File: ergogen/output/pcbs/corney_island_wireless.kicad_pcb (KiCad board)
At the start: 2 copper layers, 133.8 x 91.7 mm, 75 parts

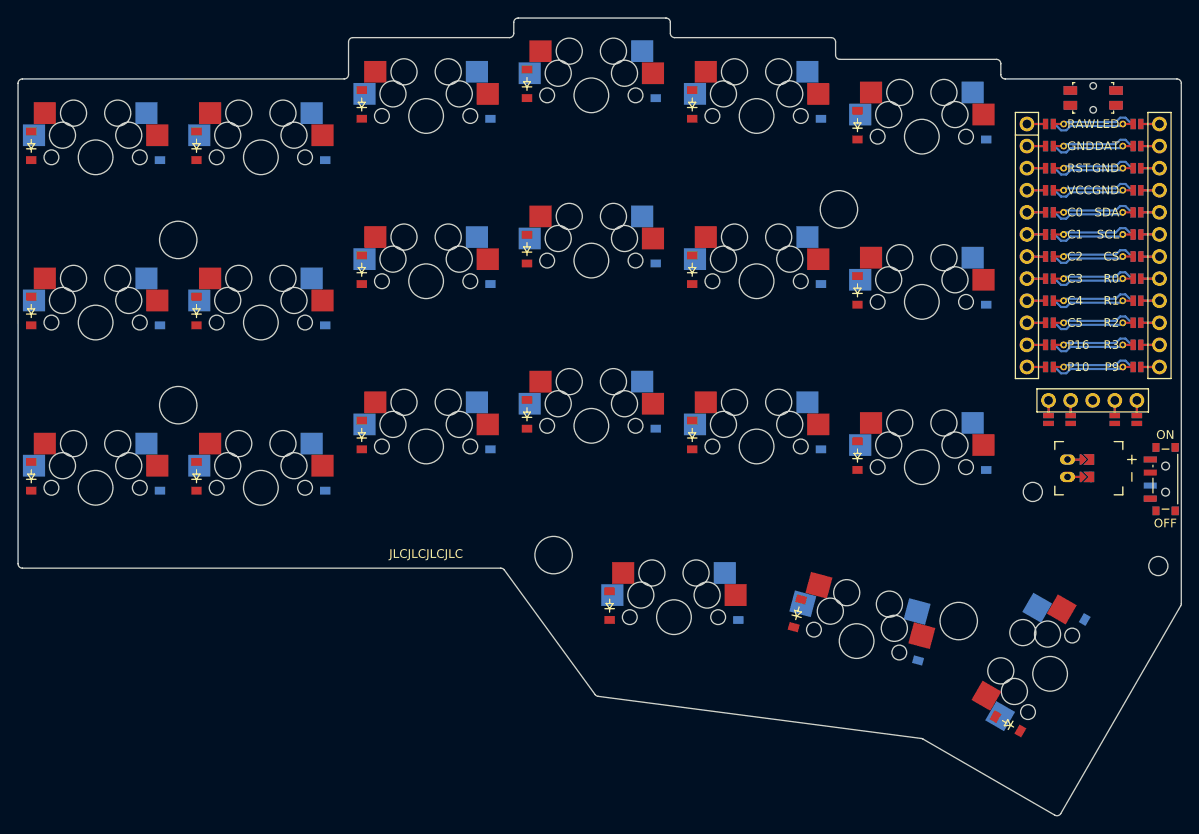
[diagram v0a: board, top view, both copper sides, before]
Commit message: Update assets
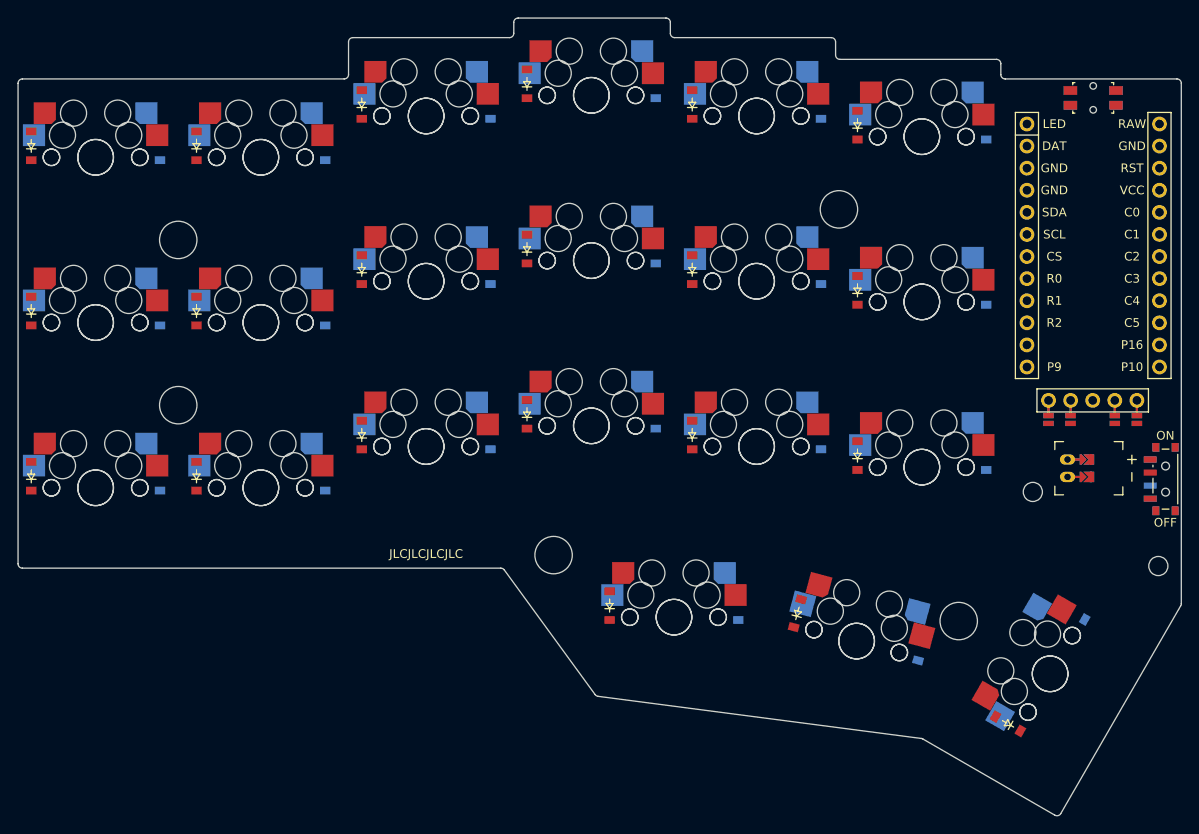
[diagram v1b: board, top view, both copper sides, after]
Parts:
- added S22: , ceoloide:switch_mx, F.Cu at (100.0, 100.0)
- added S23: , ceoloide:switch_mx, F.Cu at (100.0, 81.0)
- added S24: , ceoloide:switch_mx, F.Cu at (100.0, 62.0)
- added S25: , ceoloide:switch_mx, F.Cu at (119.0, 100.0)
- added S26: , ceoloide:switch_mx, F.Cu at (119.0, 81.0)
- added S27: , ceoloide:switch_mx, F.Cu at (119.0, 62.0)
- added S28: , ceoloide:switch_mx, F.Cu at (138.0, 95.2)
- added S29: , ceoloide:switch_mx, F.Cu at (138.0, 76.2)
- added S30: , ceoloide:switch_mx, F.Cu at (138.0, 57.2)
- added S31: , ceoloide:switch_mx, F.Cu at (157.0, 92.9)
- added S32: , ceoloide:switch_mx, F.Cu at (157.0, 73.9)
- added S33: , ceoloide:switch_mx, F.Cu at (157.0, 54.9)
- added S34: , ceoloide:switch_mx, F.Cu at (176.0, 95.2)
- added S35: , ceoloide:switch_mx, F.Cu at (176.0, 76.2)
- added S36: , ceoloide:switch_mx, F.Cu at (176.0, 57.2)
- added S37: , ceoloide:switch_mx, F.Cu at (195.0, 97.6)
- added S38: , ceoloide:switch_mx, F.Cu at (195.0, 78.6)
- added S39: , ceoloide:switch_mx, F.Cu at (195.0, 59.6)
- added S40: , ceoloide:switch_mx, F.Cu at (166.5, 114.9)
- added S41: , ceoloide:switch_mx, F.Cu at (187.5, 117.6)
- added S42: , ceoloide:switch_mx, F.Cu at (209.7, 121.4)
- PWR1: value power_switch -> (none)
- RST1: value reset_button_smd_side -> (none); footprint ceoloide:reset_button_smd_side -> ceoloide:reset_switch_smd_side
- S1, S10, S11, S12, S13, S14, S15, S16, S17, S18, S19, S2, S20, S21, S3, S4, S5, S6, S7, S8, S9: footprint MX -> ceoloide:switch_mx; moved to B.Cu
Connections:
- D1 pad 2: outer_bottom -> outer_bottom_B
- D10 pad 2: middle_bottom -> middle_bottom_B
- D11 pad 2: middle_home -> middle_home_B
- D12 pad 2: middle_top -> middle_top_B
- D13 pad 2: index_bottom -> index_bottom_B
- D14 pad 2: index_home -> index_home_B
- D15 pad 2: index_top -> index_top_B
- D16 pad 2: inner_bottom -> inner_bottom_B
- D17 pad 2: inner_home -> inner_home_B
- D18 pad 2: inner_top -> inner_top_B
- D19 pad 2: near_home -> near_home_B
- D2 pad 2: outer_home -> outer_home_B
- D20 pad 2: mid_home -> mid_home_B
- D21 pad 2: far_home -> far_home_B
- D22 pad 2: outer_bottom -> outer_bottom_F
- D23 pad 2: outer_home -> outer_home_F
- D24 pad 2: outer_top -> outer_top_F
- D25 pad 2: pinky_bottom -> pinky_bottom_F
- D26 pad 2: pinky_home -> pinky_home_F
- D27 pad 2: pinky_top -> pinky_top_F
- D28 pad 2: ring_bottom -> ring_bottom_F
- D29 pad 2: ring_home -> ring_home_F
- D3 pad 2: outer_top -> outer_top_B
- D30 pad 2: ring_top -> ring_top_F
- D31 pad 2: middle_bottom -> middle_bottom_F
- D32 pad 2: middle_home -> middle_home_F
- D33 pad 2: middle_top -> middle_top_F
- D34 pad 2: index_bottom -> index_bottom_F
- D35 pad 2: index_home -> index_home_F
- D36 pad 2: index_top -> index_top_F
- D37 pad 2: inner_bottom -> inner_bottom_F
- D38 pad 2: inner_home -> inner_home_F
- D39 pad 2: inner_top -> inner_top_F
- D4 pad 2: pinky_bottom -> pinky_bottom_B
- D40 pad 2: near_home -> near_home_F
- D41 pad 2: mid_home -> mid_home_F
- D42 pad 2: far_home -> far_home_F
- D5 pad 2: pinky_home -> pinky_home_B
- D6 pad 2: pinky_top -> pinky_top_B
- D7 pad 2: ring_bottom -> ring_bottom_B
- D8 pad 2: ring_home -> ring_home_B
- D9 pad 2: ring_top -> ring_top_B
- MCU1 pad 1: MCU1_1 -> RAW
- MCU1 pad 10: MCU1_10 -> C5
- MCU1 pad 11: MCU1_11 -> P16
- MCU1 pad 12: MCU1_12 -> P10
- MCU1 pad 13: MCU1_12 -> P9
- MCU1 pad 14: MCU1_11 -> R3
- MCU1 pad 15: MCU1_10 -> R2
- MCU1 pad 16: MCU1_9 -> R1
- MCU1 pad 17: MCU1_8 -> R0
- MCU1 pad 18: MCU1_7 -> CS
- MCU1 pad 19: MCU1_6 -> SCL
- MCU1 pad 2: MCU1_2 -> GND
- MCU1 pad 20: MCU1_5 -> SDA
- MCU1 pad 21: MCU1_4 -> GND
- MCU1 pad 22: MCU1_3 -> GND
- MCU1 pad 23: MCU1_2 -> DAT
- MCU1 pad 24: MCU1_1 -> LED
- MCU1 pad 3: MCU1_3 -> RST
- MCU1 pad 4: MCU1_4 -> VCC
- MCU1 pad 5: MCU1_5 -> C0
- MCU1 pad 6: MCU1_6 -> C1
- MCU1 pad 7: MCU1_7 -> C2
- MCU1 pad 8: MCU1_8 -> C3
- MCU1 pad 9: MCU1_9 -> C4
- S1 pad 2: outer_bottom -> outer_bottom_B
- S10 pad 2: middle_bottom -> middle_bottom_B
- S11 pad 2: middle_home -> middle_home_B
- S12 pad 2: middle_top -> middle_top_B
- S13 pad 2: index_bottom -> index_bottom_B
- S14 pad 2: index_home -> index_home_B
- S15 pad 2: index_top -> index_top_B
- S16 pad 2: inner_bottom -> inner_bottom_B
- S17 pad 2: inner_home -> inner_home_B
- S18 pad 2: inner_top -> inner_top_B
- S19 pad 2: near_home -> near_home_B
- S2 pad 2: outer_home -> outer_home_B
- S20 pad 2: mid_home -> mid_home_B
- S21 pad 2: far_home -> far_home_B
- S3 pad 2: outer_top -> outer_top_B
- S4 pad 2: pinky_bottom -> pinky_bottom_B
- S5 pad 2: pinky_home -> pinky_home_B
- S6 pad 2: pinky_top -> pinky_top_B
- S7 pad 2: ring_bottom -> ring_bottom_B
- S8 pad 2: ring_home -> ring_home_B
- S9 pad 2: ring_top -> ring_top_B
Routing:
- net GND: track 28.9 -> 0.00 mm
- net C3: track 9.64 -> 0.00 mm
- net C1: track 9.64 -> 0.00 mm
- net VCC: track 9.64 -> 0.00 mm
- net RST: track 9.64 -> 0.00 mm
- net RAW: track 9.64 -> 0.00 mm
- net C4: track 9.64 -> 0.00 mm
- net C2: track 9.64 -> 0.00 mm
- net C0: track 9.64 -> 0.00 mm
- net P16: track 9.64 -> 0.00 mm
- net P10: track 9.64 -> 0.00 mm
- net C5: track 9.64 -> 0.00 mm
- net SDA: track 9.63 -> 0.00 mm
- net R3: track 9.63 -> 0.00 mm
- net R1: track 9.63 -> 0.00 mm
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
